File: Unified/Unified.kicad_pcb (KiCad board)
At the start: 2 copper layers, 72.4 x 72.4 mm, 55 parts, among them J1 USB_C_Receptacle_USB2.0_16P, J10 JST_switch_1, J11 JST_switch_2, J12 Conn_touch_1, J13 Conn_touch_2, J14 Bat_pos_sel, J15 Bat_neg_sel, J2 JST_battery, J3 JST_header, J4 JST_speaker, J5 JST_debug_swd, J6 JST_debug_serial, J7 Conn_speaker_sd, J8 Conn_speaker_gain, J9 Conn_speaker_gnd, Q1 AO3401A, Q2 AO3400A, SW1 SW_power, U1 MCP73831-2-OT, U2 MAX98357A

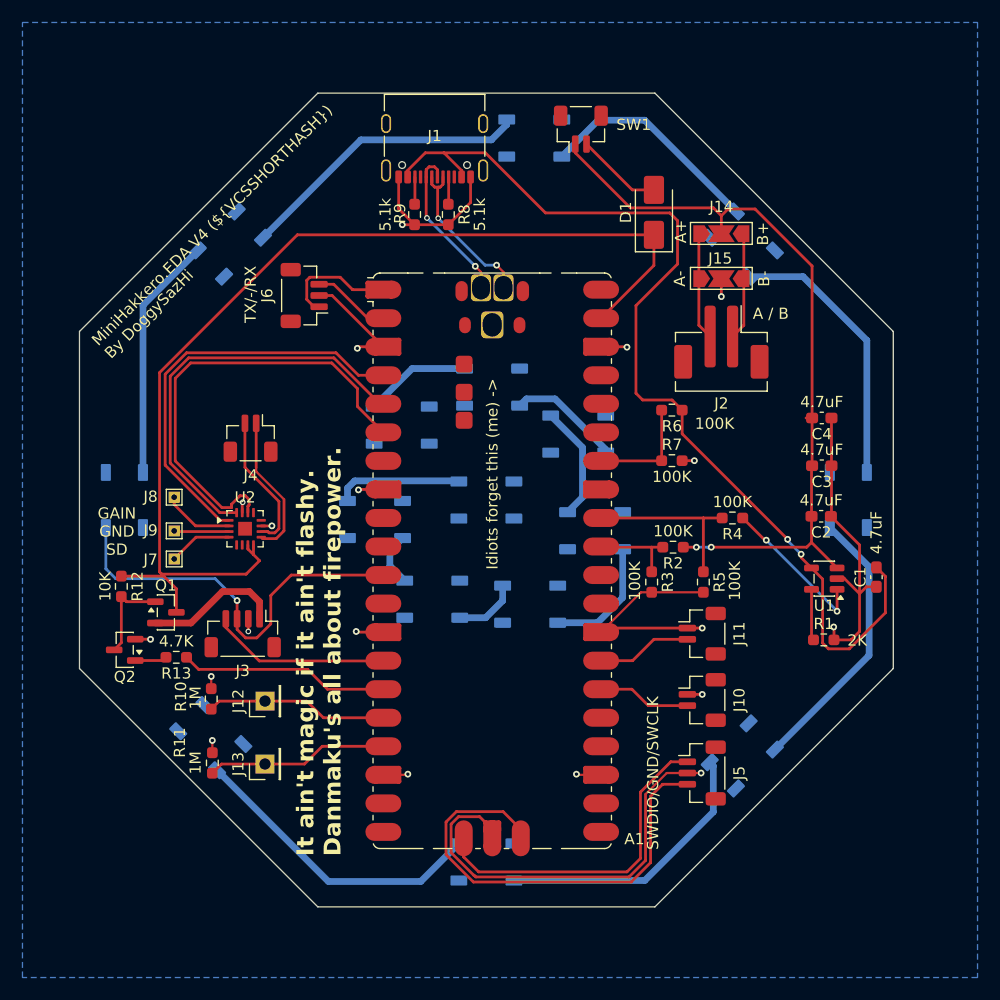
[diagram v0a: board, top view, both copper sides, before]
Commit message: Try to route but Kicad decided to crash
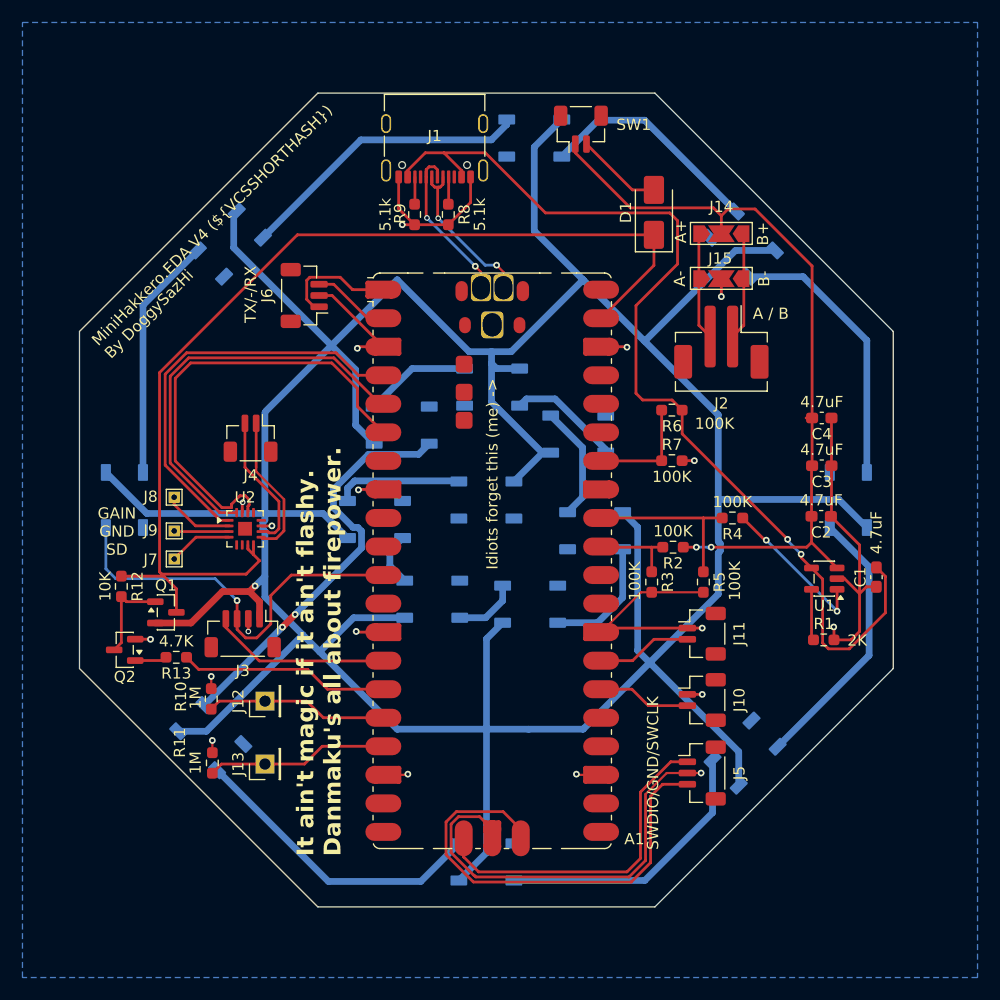
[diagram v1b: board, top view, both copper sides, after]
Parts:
- moved D7 0.35 mm to (179.3, 125.0)
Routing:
- net /WS2812B_VS: track 12.3 -> 343.4 mm, vias 0 -> 1
- net Net-(D10-DIN): track 0.00 -> 36.5 mm, vias 0 -> 2
